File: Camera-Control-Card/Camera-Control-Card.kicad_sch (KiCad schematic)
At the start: 1 part, among them J2 Conn_01x10

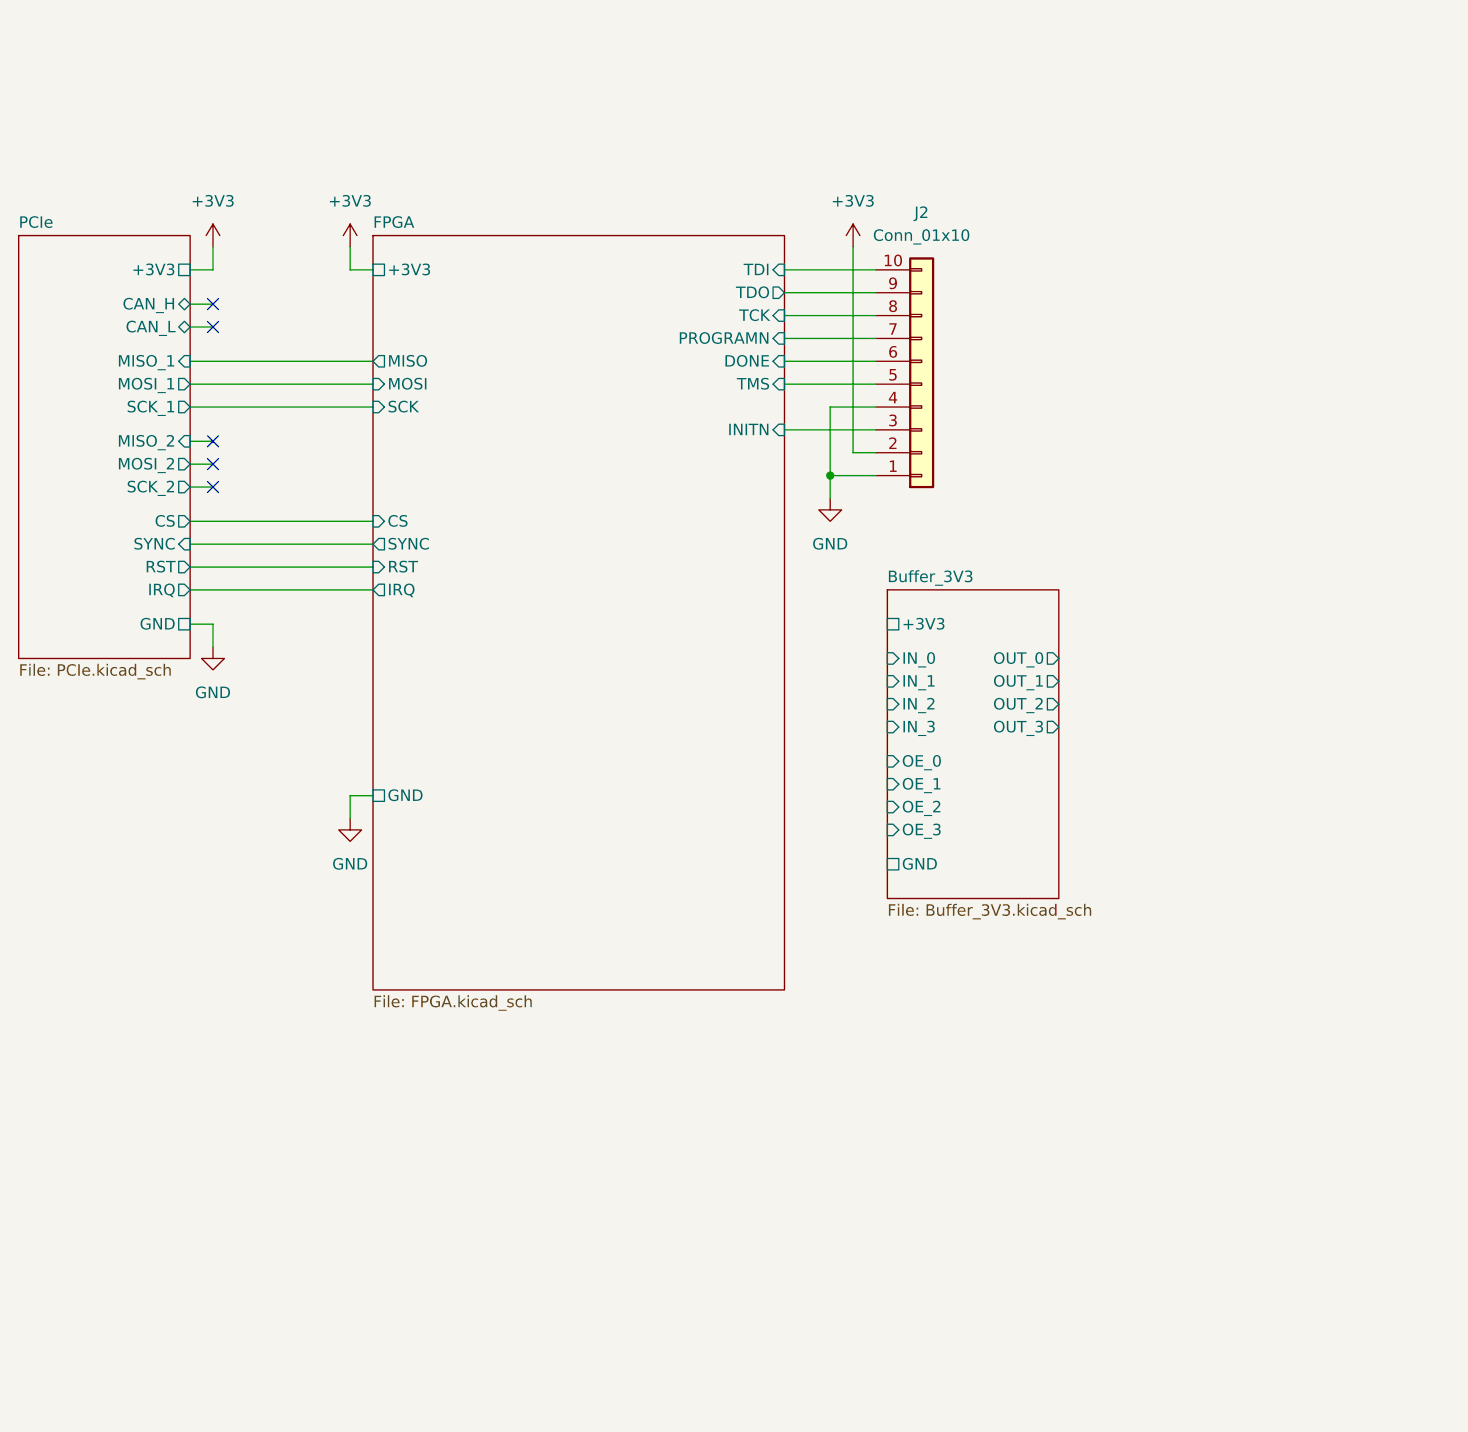
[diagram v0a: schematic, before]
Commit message: test
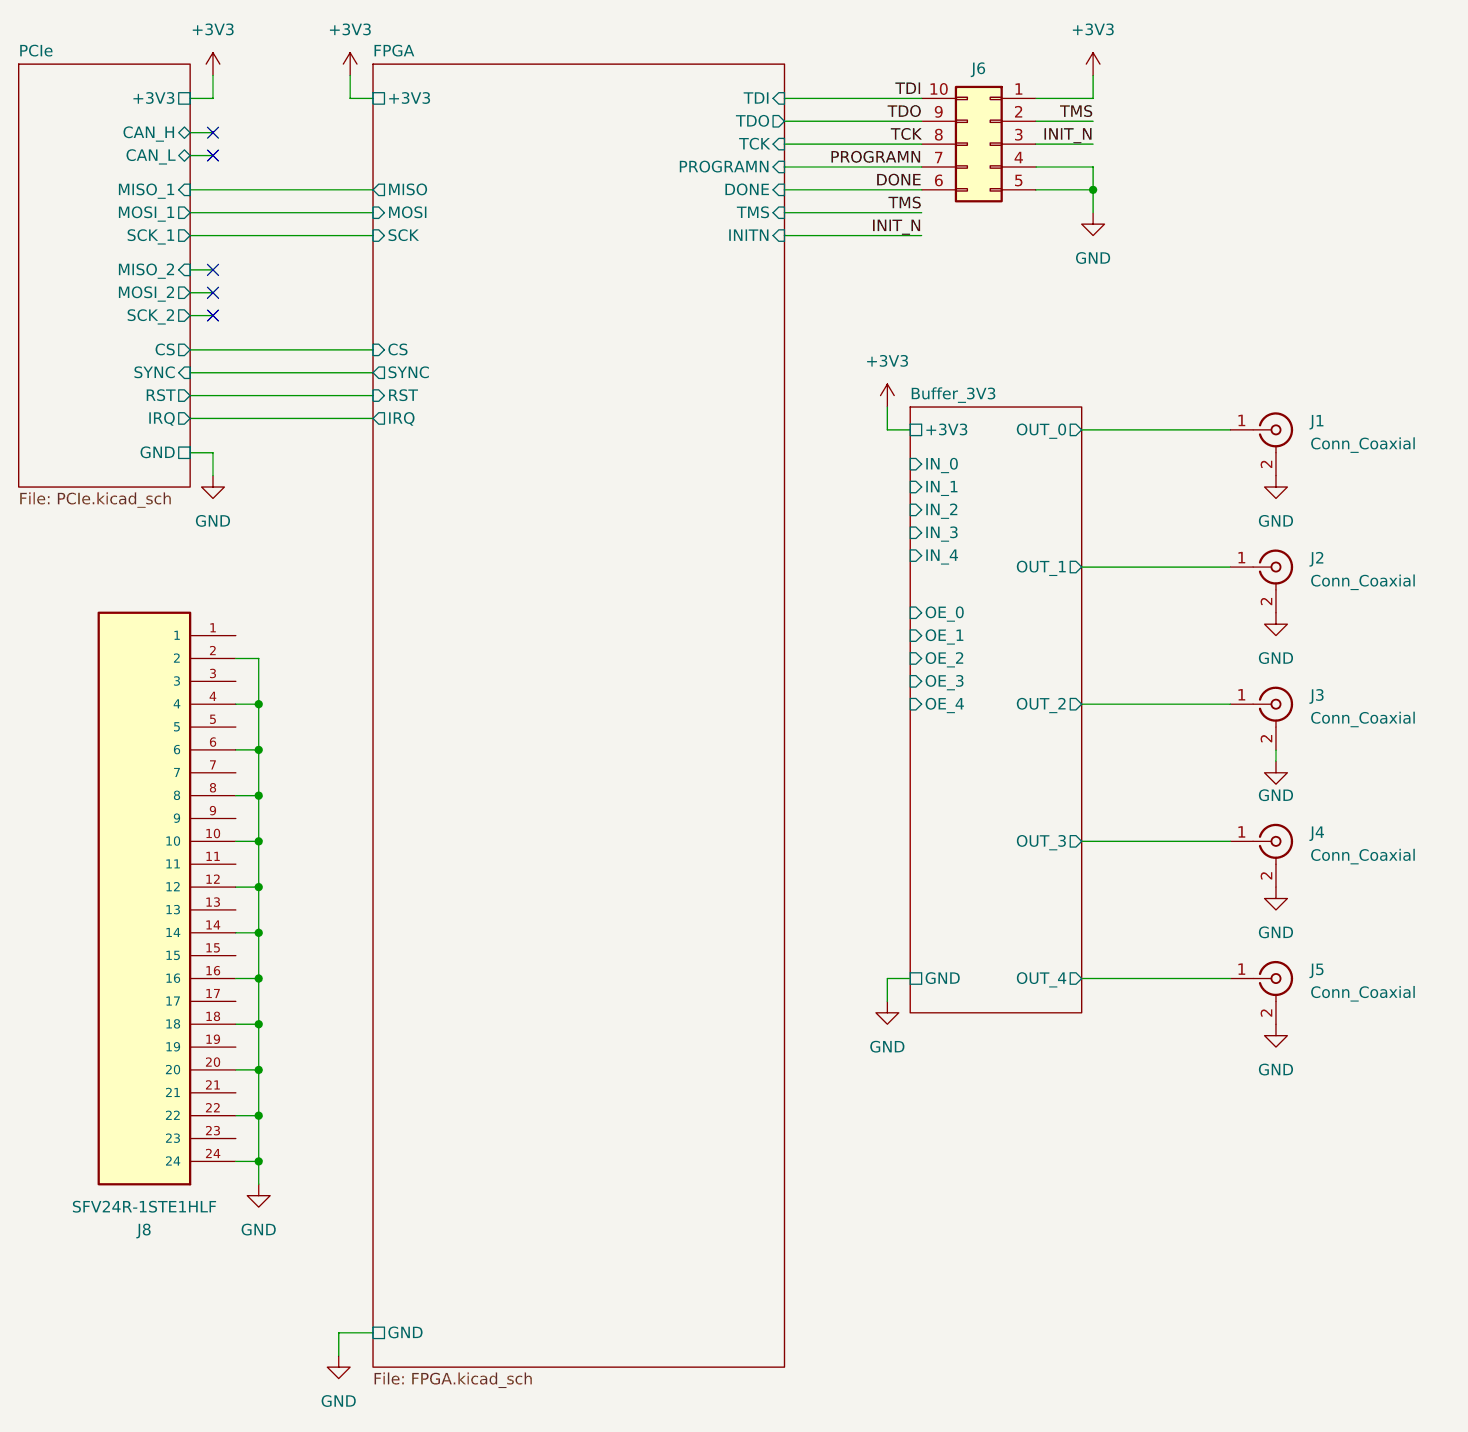
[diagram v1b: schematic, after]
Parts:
- removed J2: Conn_01x10, Connector_PinHeader_2.54mm:PinHeader_2x05_P2.54mm_Vertical, symbol Connector_Generic:Conn_01x10
- added J1, J2, J3, J4, J5: Conn_Coaxial, Connector_Coaxial:SMA_Molex_73251-1153_EdgeMount_Horizontal, symbol Connector:Conn_Coaxial
- added J6: Conn_02x05_Counter_Clockwise, symbol Connector_Generic:Conn_02x05_Counter_Clockwise
- added J8: SFV24R-1STE1HLF, Footprints:AMPHENOL_SFV24R-1STE1HLF, symbol Symbols:SFV24R-1STE1HLF
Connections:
- net +3V3: now also J6.1 (Pin_1)
- net Buffer_3V3/OUT_0: now also J1.1 (In)
- net Buffer_3V3/OUT_1: now also J2.1 (In)
- net Buffer_3V3/OUT_2: now also J3.1 (In)
- net Buffer_3V3/OUT_3: now also J4.1 (In)
- net GND: now also J1.2 (Ext), J2.2 (Ext), J3.2 (Ext), J4.2 (Ext), J5.2 (Ext), J6.4 (Pin_4), J6.5 (Pin_5), J8.10, J8.12, J8.14, J8.16, J8.18, J8.2, J8.20, J8.22, J8.24, J8.4, J8.6, J8.8
- new net Buffer_3V3/OUT_4: J5.1 (In)
- new net DONE: J6.6 (Pin_6)
- new net INIT_N: J6.3 (Pin_3)
- new net PROGRAMN: J6.7 (Pin_7)
- new net TCK: J6.8 (Pin_8)
- new net TDI: J6.10 (Pin_10)
- new net TDO: J6.9 (Pin_9)
- new net TMS: J6.2 (Pin_2)
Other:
- sheet Buffer_3V3 ports: added IN_4, OE_4, OUT_4; removed none
